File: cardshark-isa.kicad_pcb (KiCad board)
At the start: 4 copper layers, 153.5 x 82.1 mm, 98 parts, among them J1 Conn_02x13_Odd_Even, J3 DE15_Receptacle_HighDensity_M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, J4 Bus_ISA_16bit, U1 GD543x_ISA, U11 93CxxA, U12 SOJ_256Kx16, U13 SOJ_256Kx16, U2 27C256, U3 SOJ_256Kx16, U5 74AHCT1G04, U6 SN74LS245DBR, U7 SOJ_256Kx16, U9 LM334M

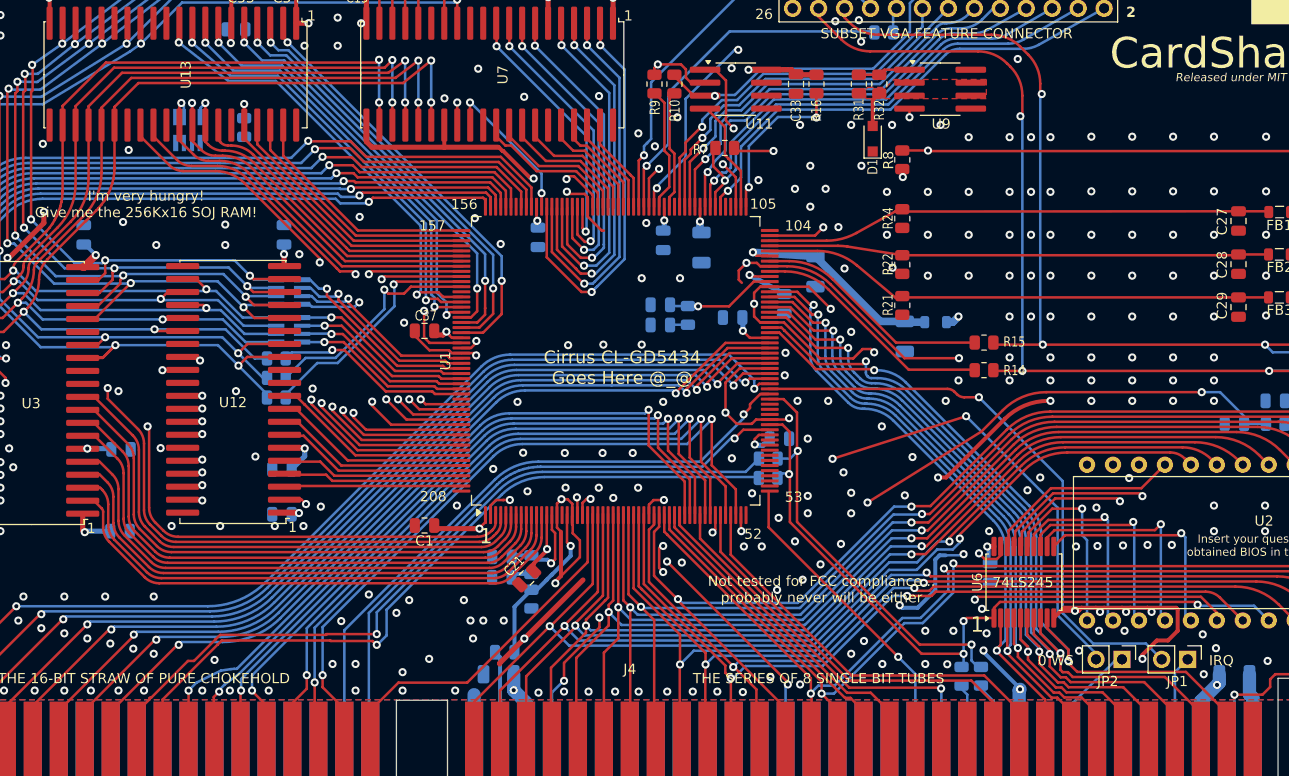
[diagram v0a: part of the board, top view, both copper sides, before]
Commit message: Add files via upload
Uploaded CSV BOM. Made various little, very minor quick fixes, mostly of a cosmetic nature.
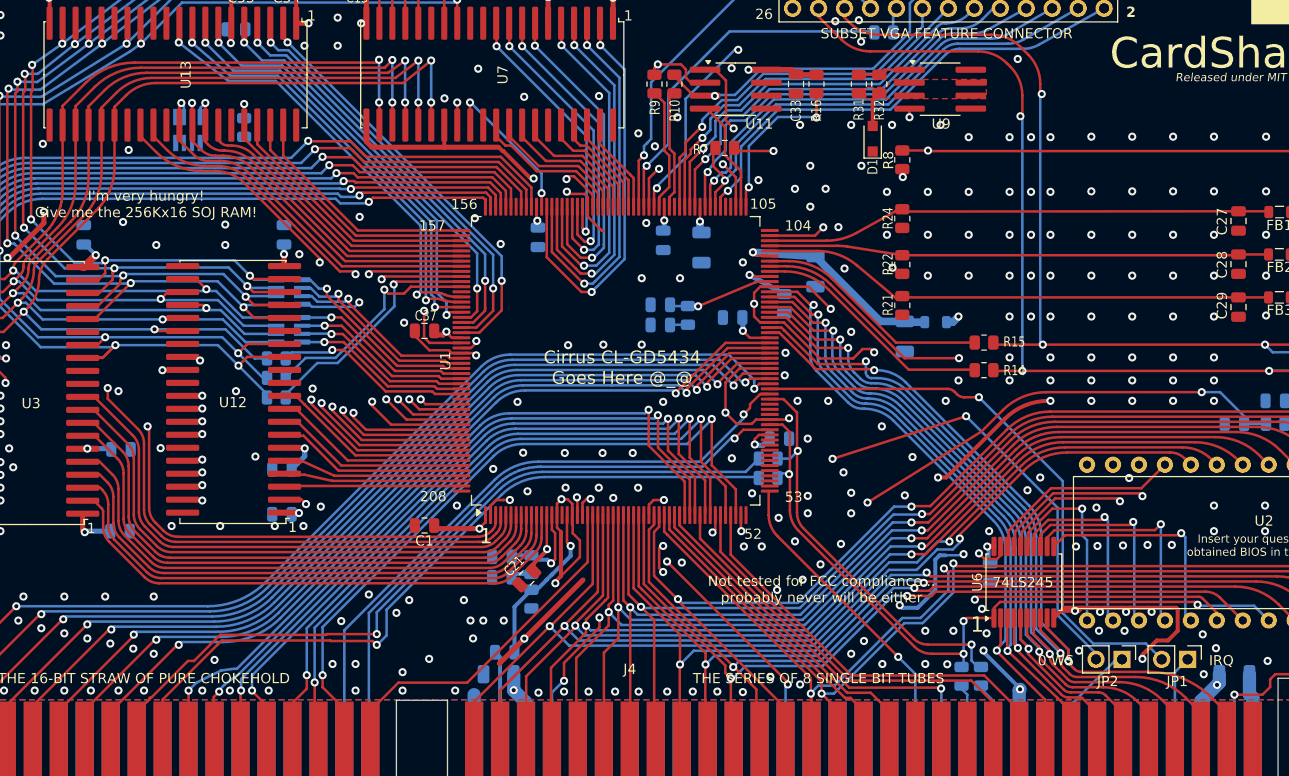
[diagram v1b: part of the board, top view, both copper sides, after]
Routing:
- net GND: track 257.1 -> 252.4 mm
- net /SD6: track 70.0 -> 69.2 mm
- net /SD5: track 67.7 -> 67.0 mm
- net /SD4: track 65.4 -> 64.7 mm
- net /VFILTER: track 10.8 -> 10.3 mm
